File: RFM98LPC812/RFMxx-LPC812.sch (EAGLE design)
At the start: 21 parts, among them X1 BU-SMA-V, X2 BU-SMA-V

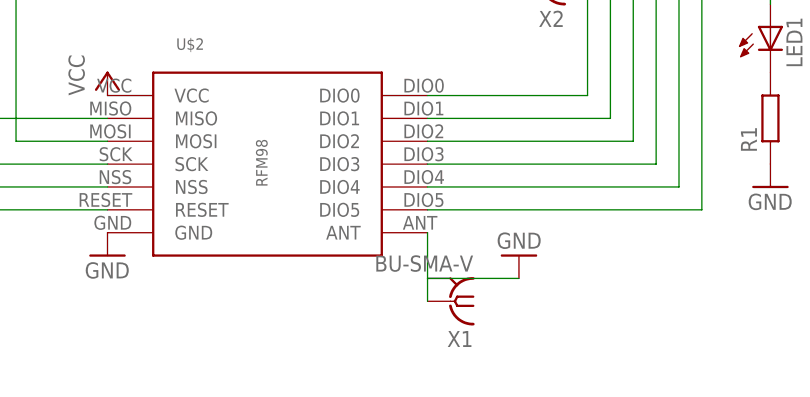
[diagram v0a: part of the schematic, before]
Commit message: no comment
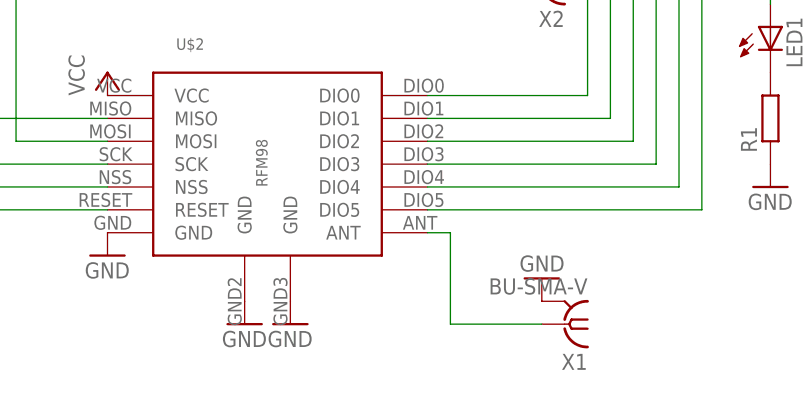
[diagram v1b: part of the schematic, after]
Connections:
- new net N$26: R1.1, R2.1, R3.1, R4.1, R5.1, R6.1, U$1.VSS, U$2.GND, U$2.GND@2, U$2.GND@3, U$3.GND, U$4.-, X2.2
- net GND: no longer R1.1, R2.1, R3.1, R4.1, R5.1, R6.1, U$1.VSS, U$2.GND, U$3.GND, U$4.-, X2.2
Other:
- moved on the sheet: X1
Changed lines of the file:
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@@
 <part name="P+3" library="supply1" deviceset="VCC" device=""/>
 <part name="P+4" library="supply1" deviceset="VCC" device=""/>
+<part name="GND13" library="supply1" deviceset="GND" device=""/>
+<part name="GND14" library="supply1" deviceset="GND" device=""/>
 </parts>
 <sheets>
@@
 <instances>
 <instance part="U$2" gate="G$1" x="0" y="2.54"/>
-<instance part="X1" gate="G$1" x="20.32" y="-10.16" rot="R180"/>
+<instance part="X1" gate="G$1" x="33.02" y="-12.7" rot="R180"/>
 <instance part="X2" gate="G$1" x="30.48" y="25.4" rot="R180"/>
 <instance part="JP1" gate="A" x="-43.18" y="40.64"/>
@@
 <instance part="GND2" gate="1" x="-101.6" y="68.58" rot="R180"/>
 <instance part="GND3" gate="1" x="27.94" y="30.48" rot="R180"/>
-<instance part="GND4" gate="1" x="27.94" y="-5.08" rot="R180"/>
+<instance part="GND4" gate="1" x="30.48" y="-7.62" rot="R180"/>
 <instance part="GND5" gate="1" x="55.88" y="2.54"/>
 <instance part="GND6" gate="1" x="66.04" y="2.54"/>
@@
 <instance part="P+3" gate="VCC" x="-17.78" y="48.26"/>
 <instance part="P+4" gate="VCC" x="-17.78" y="15.24"/>
+<instance part="GND13" gate="1" x="-2.54" y="-12.7"/>
+<instance part="GND14" gate="1" x="2.54" y="-12.7"/>
 </instances>
 <busses>
@@
 <wire x1="17.78" y1="30.48" x2="27.94" y2="25.4" width="0.1524" layer="91"/>
 <pinref part="U$3" gate="G$1" pin="ANT"/>
-</segment>
-</net>
-<net name="N$6" class="0">
-<segment>
-<pinref part="U$2" gate="G$1" pin="ANT"/>
-<pinref part="X1" gate="G$1" pin="1"/>
-<wire x1="17.78" y1="-2.54" x2="17.78" y2="-10.16" width="0.1524" layer="91"/>
 </segment>
 </net>
@@
 </segment>
 </net>
-<net name="GND" class="0">
+<net name="N$26" class="0">
 <segment>
 <pinref part="U$4" gate="G$1" pin="-"/>
@@
 </segment>
 <segment>
-<pinref part="X1" gate="G$1" pin="2"/>
-<pinref part="GND4" gate="1" pin="GND"/>
-<wire x1="17.78" y1="-7.62" x2="27.94" y2="-7.62" width="0.1524" layer="91"/>
-</segment>
-<segment>
 <pinref part="R1" gate="G$1" pin="1"/>
 <pinref part="GND5" gate="1" pin="GND"/>
@@
 <pinref part="U$3" gate="G$1" pin="GND"/>
 <pinref part="GND12" gate="1" pin="GND"/>
+</segment>
+<segment>
+<pinref part="U$2" gate="G$1" pin="GND@2"/>
+<pinref part="GND13" gate="1" pin="GND"/>
+</segment>
+<segment>
+<pinref part="U$2" gate="G$1" pin="GND@3"/>
+<pinref part="GND14" gate="1" pin="GND"/>
 </segment>
 </net>
@@
 </segment>
 </net>
+<net name="GND" class="0">
+<segment>
+<pinref part="X1" gate="G$1" pin="2"/>
+<pinref part="GND4" gate="1" pin="GND"/>
+</segment>
+</net>
+<net name="N$6" class="0">
+<segment>
+<pinref part="U$2" gate="G$1" pin="ANT"/>
+<wire x1="17.78" y1="-2.54" x2="20.32" y2="-2.54" width="0.1524" layer="91"/>
+<wire x1="20.32" y1="-2.54" x2="20.32" y2="-12.7" width="0.1524" layer="91"/>
+<pinref part="X1" gate="G$1" pin="1"/>
+<wire x1="20.32" y1="-12.7" x2="30.48" y2="-12.7" width="0.1524" layer="91"/>
+</segment>
+</net>
